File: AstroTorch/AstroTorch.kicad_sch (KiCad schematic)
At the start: 5 parts, among them U1 MCP1703Ax-330xxTT, U2 ATtiny24A-SS

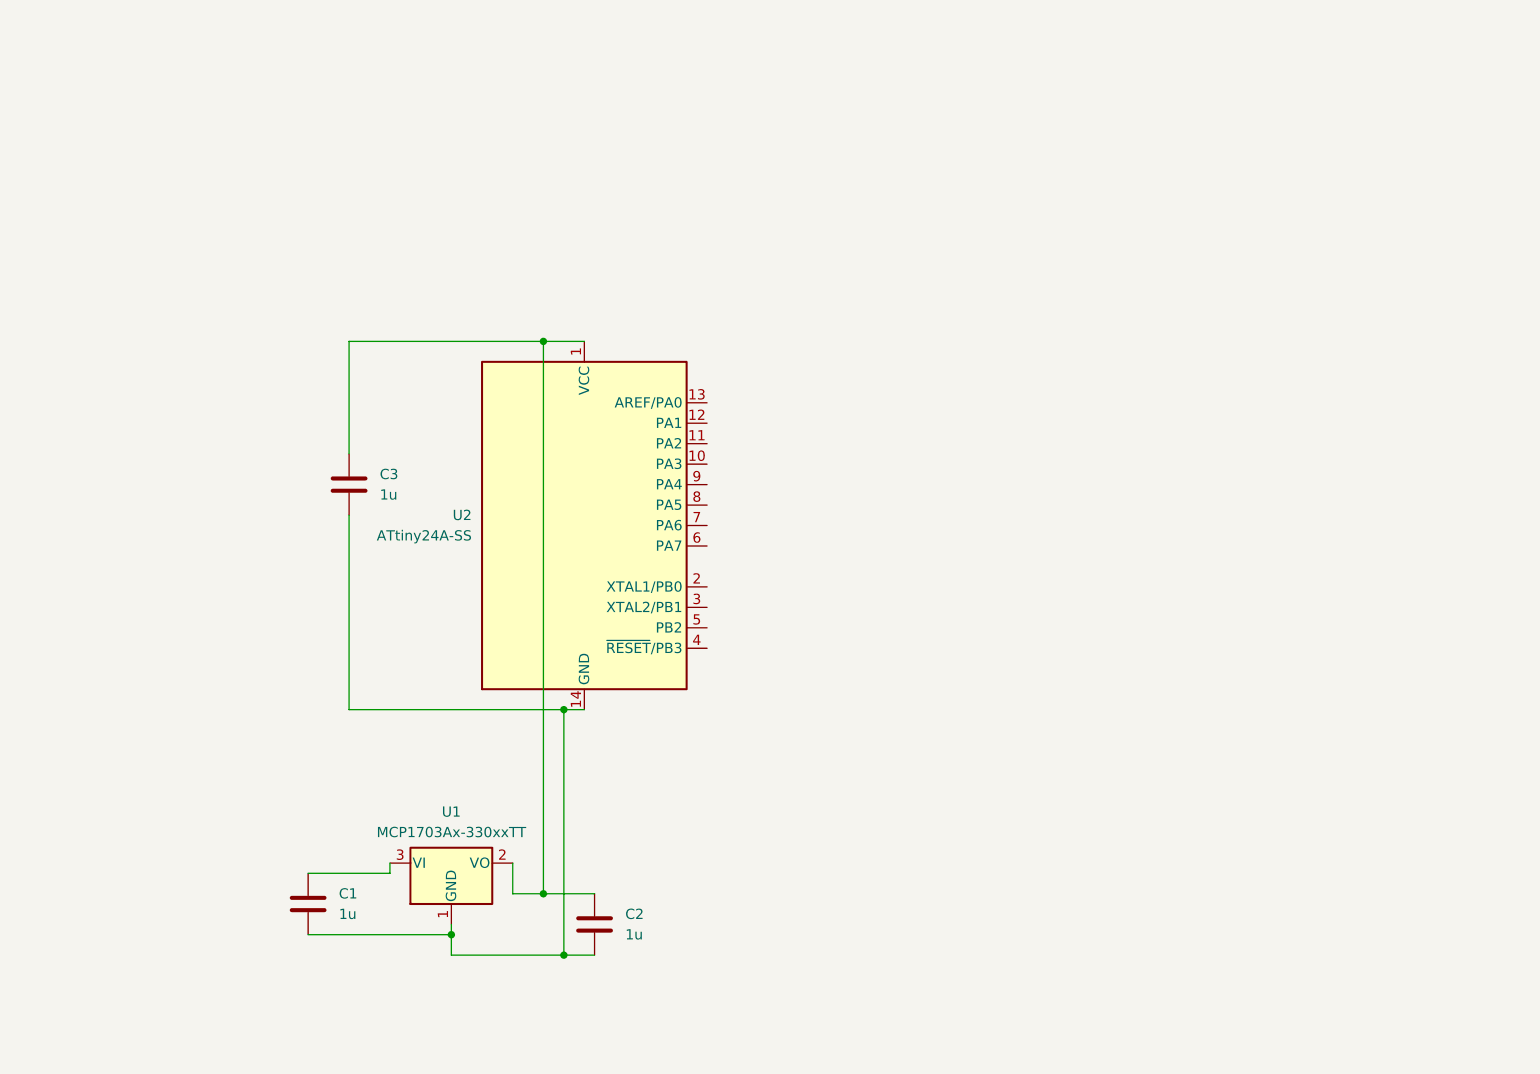
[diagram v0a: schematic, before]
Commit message: Next version
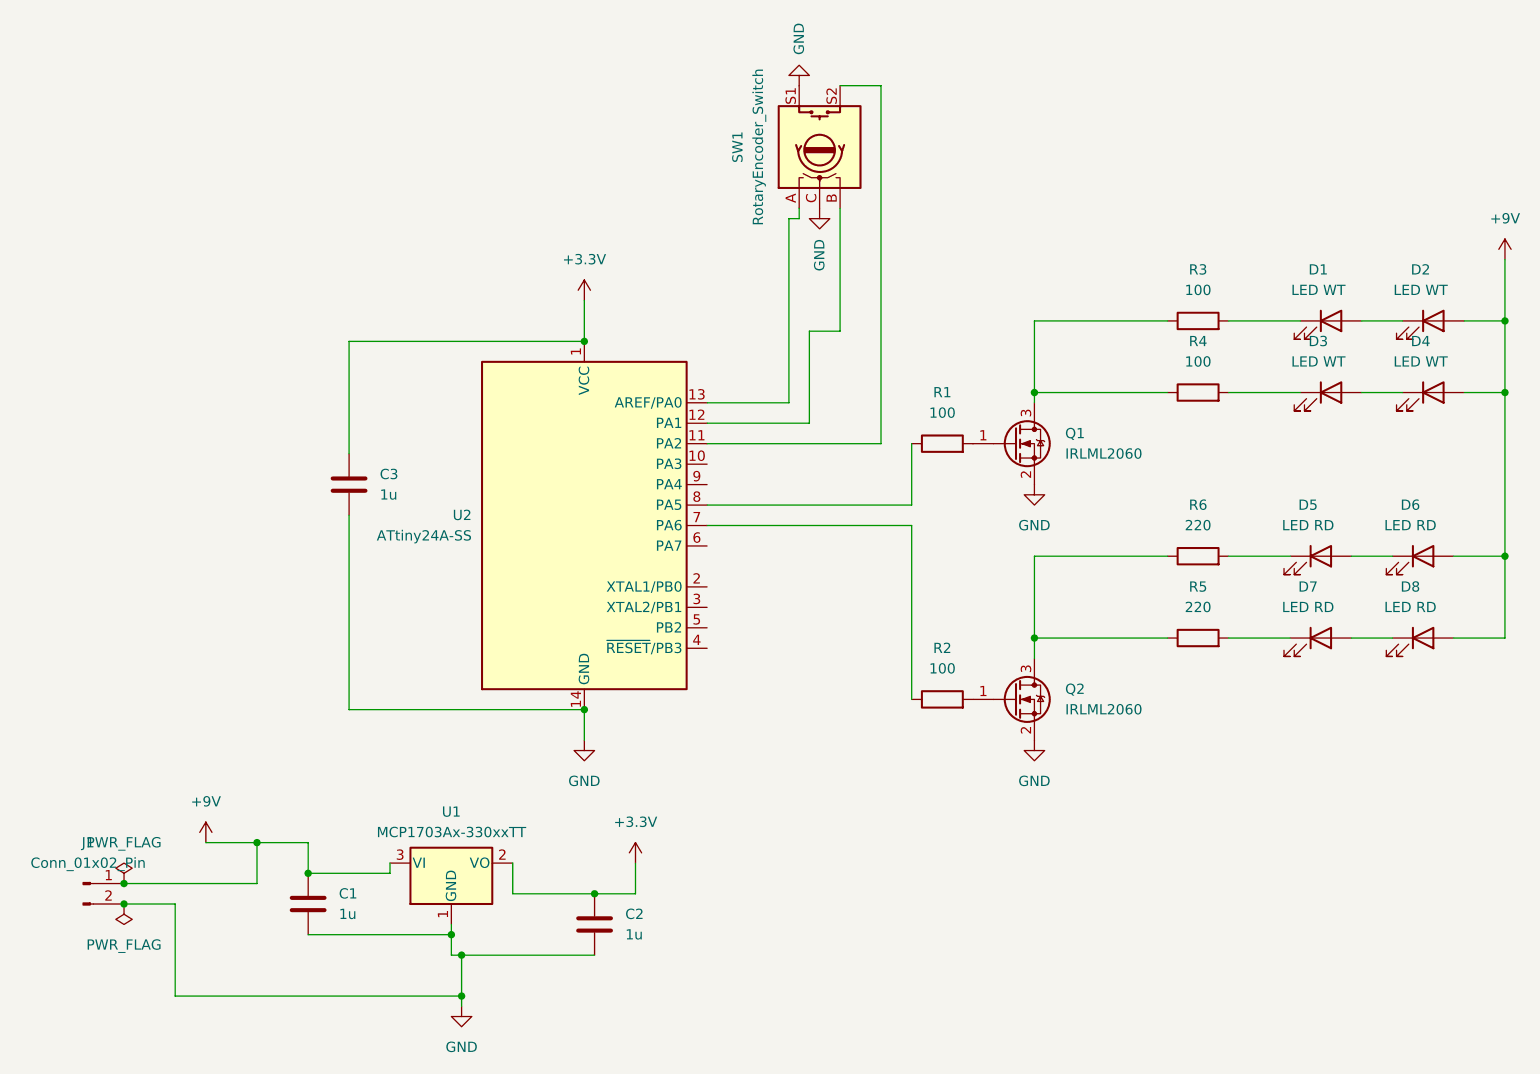
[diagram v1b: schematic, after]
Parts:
- added D1, D2, D3, D4: LED WT, LED_THT:LED_D5.0mm, symbol Device:LED
- added D5, D6, D7, D8: LED RD, LED_THT:LED_D5.0mm, symbol Device:LED
- added J1: Conn_01x02_Pin, Connector_PinHeader_2.54mm:PinHeader_1x02_P2.54mm_Vertical, symbol Connector:Conn_01x02_Pin
- added Q1, Q2: IRLML2060, Package_TO_SOT_SMD:SOT-23, symbol Transistor_FET:IRLML2060
- added R1, R2, R3, R4: 100, Resistor_SMD:R_0805_2012Metric, symbol Device:R
- added R5, R6: 220, Resistor_SMD:R_0805_2012Metric, symbol Device:R
- added SW1: RotaryEncoder_Switch, Rotary_Encoder:RotaryEncoder_Alps_EC11E-Switch_Vertical_H20mm, symbol Device:RotaryEncoder_Switch
- C1, C2, C3: footprint 0805 -> Capacitor_SMD:C_0805_2012Metric
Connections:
- net +3.3V: now reaches C2.1, C3.1, U1.2 (VO), U2.1 (VCC)
- net at U2.11 (PA2): now also SW1.S2
- net at U2.12 (PA1): now also SW1.B
- net at U2.13 (AREF/PA0): now also SW1.A
- net GND: now reaches C1.2, C2.2, C3.2, U1.1 (GND), U2.14 (GND)
- net GND: now also J1.2 (Pin_2), Q1.2 (S), Q2.2 (S), SW1.C, SW1.S1
- net at U2.7 (PA6): now also R2.1
- net at U2.8 (PA5): now also R1.1
- net +9V: now reaches C1.1, U1.3 (VI)
- net +9V: now also D2.2 (A), D4.2 (A), D6.2 (A), D8.2 (A), J1.1 (Pin_1)
- new net: D3.2 (A), D4.1 (K)
- new net: Q1.1 (G), R1.2
- new net: Q1.3 (D), R3.1, R4.1
- new net: D5.1 (K), R6.2
- new net: D5.2 (A), D6.1 (K)
- new net: D1.2 (A), D2.1 (K)
- new net: D1.1 (K), R3.2
- new net: Q2.3 (D), R5.1, R6.1
- new net: D7.1 (K), R5.2
- new net: D7.2 (A), D8.1 (K)
- new net: Q2.1 (G), R2.2
- new net: D3.1 (K), R4.2
